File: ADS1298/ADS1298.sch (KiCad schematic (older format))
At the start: 269 parts, among them IC1 ADS1298, IC2 ADuM6401, IC3 ADuM4401, IC4 ADM811, IC5 REF5025, IC6 OPA211, P1 ADS_Sensors, P2 PCB_BoardCut, U1 ADS1298_Control, U2 TPS79230, U3 TPS79101, U4 TPS60403, U5 TPS72325

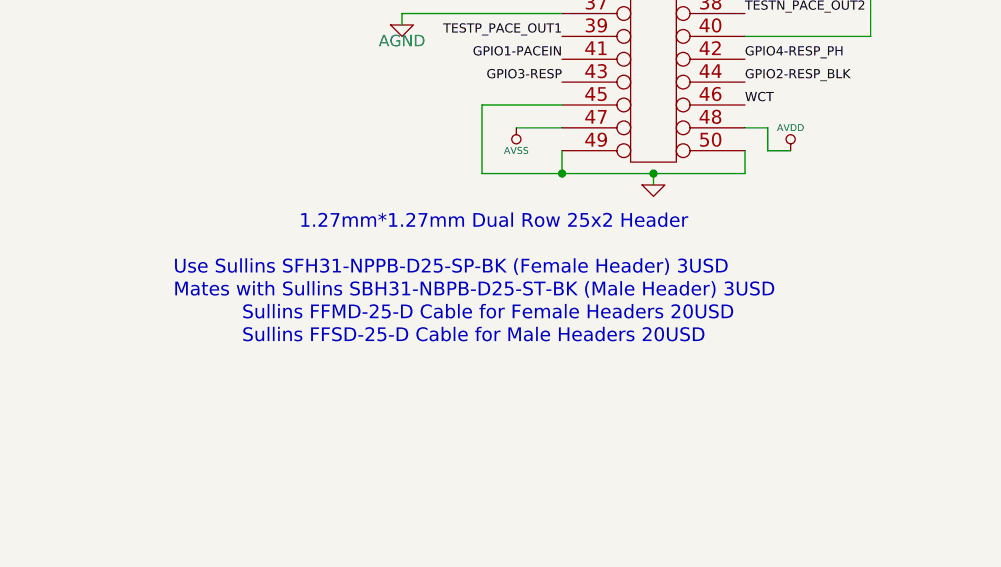
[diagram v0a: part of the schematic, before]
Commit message: Minor update to ADS1298 project.
git-svn-id: http://opendous.googlecode.com/svn/trunk/Current_Designs@189 3806c4c6-82b1-11dd-ad27-0f66e57d2035
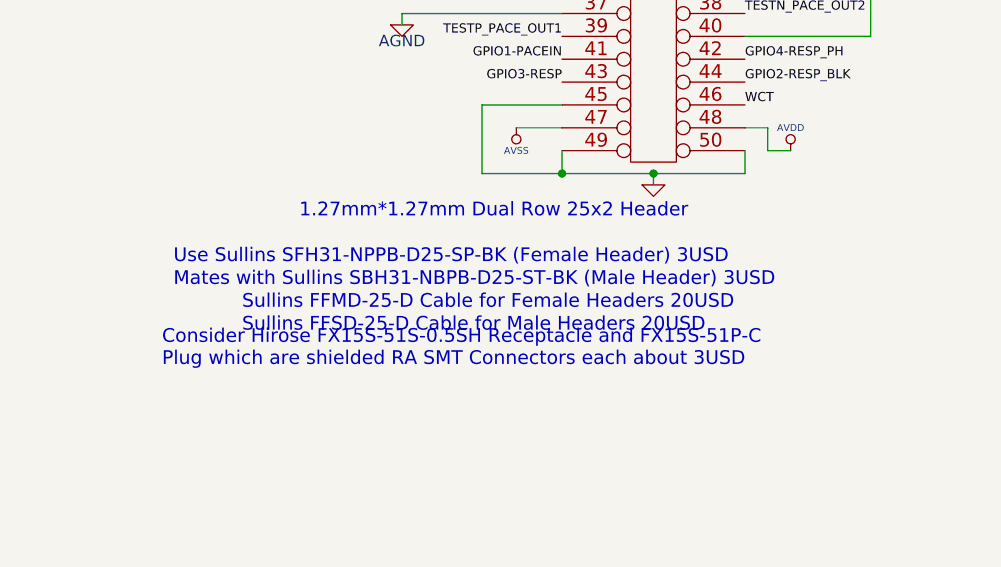
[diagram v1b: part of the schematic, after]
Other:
- note added: "Consider Hirose FX15S-51S-0.5SH Receptacle and FX15S-51P-C\nPlug which are shielded RA SMT Connectors each about 3USD"
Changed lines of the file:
@@
-EESchema Schematic File Version 2  date 17/04/2010 17:11:51
+EESchema Schematic File Version 2  date 18/04/2010 02:44:13
 LIBS:opendous
 LIBS:device
@@
 Sheet 1 1
 Title "ADS1298 Base Board"
-Date "17 apr 2010"
+Date "18 apr 2010"
 Rev "1.0"
 Comp "Opendous Inc. (www.opendous.org)"
@@
 Comment4 "http://www.opendous.org/BioSensorPlatform"
 $EndDescr
+Text Notes 8050 6450 0    60   ~ 0
+Consider Hirose FX15S-51S-0.5SH Receptacle and FX15S-51P-C\nPlug which are shielded RA SMT Connectors each about 3USD
 Text Notes 1950 1650 0    30   ~ 0
 GND Fence surrounds\ncircuit to limit EMI
@@
 	0    1    1    0
 $EndComp
-Text Notes 8400 6250 0    60   ~ 0
+Text Notes 8400 6200 0    60   ~ 0
 Sullins FFMD-25-D Cable for Female Headers 20USD
-Text Notes 8400 6350 0    60   ~ 0
+Text Notes 8400 6300 0    60   ~ 0
 Sullins FFSD-25-D Cable for Male Headers 20USD
-Text Notes 8100 6050 0    60   ~ 0
+Text Notes 8100 6000 0    60   ~ 0
 Use Sullins SFH31-NPPB-D25-SP-BK (Female Header) 3USD
 Text Label 2000 6250 0    20   ~ 0
@@
 Text Notes 5450 550  0    40   ~ 0
 CLKSEL=0 for External Clock\nCLKSEL=1 for Internal Clock\nas per datasheet Pg24
-Text Notes 8100 6150 0    60   ~ 0
+Text Notes 8100 6100 0    60   ~ 0
 Mates with Sullins SBH31-NBPB-D25-ST-BK (Male Header) 3USD
 Text Notes 1850 2850 0    40   ~ 0
@@
 Text Notes 3500 3400 0    60   ~ 0
 DVDD
-Text Notes 8650 5850 0    60   ~ 0
+Text Notes 8650 5800 0    60   ~ 0
 1.27mm*1.27mm Dual Row 25x2 Header
 $Comp
